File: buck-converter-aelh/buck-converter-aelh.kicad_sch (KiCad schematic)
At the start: 28 parts

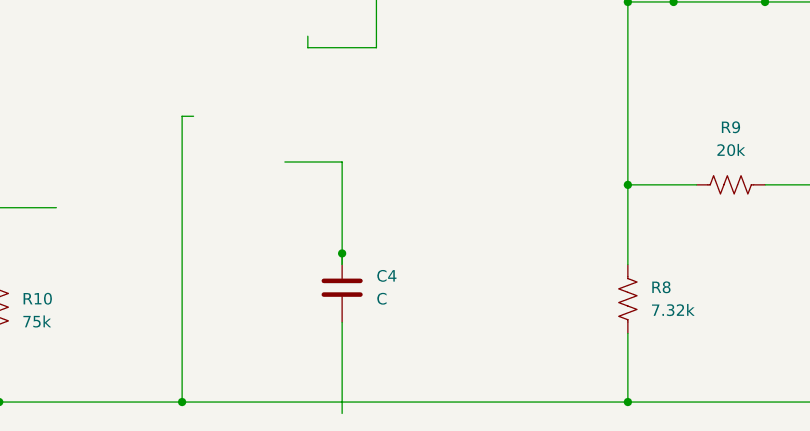
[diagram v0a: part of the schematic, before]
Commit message: AELH symbol
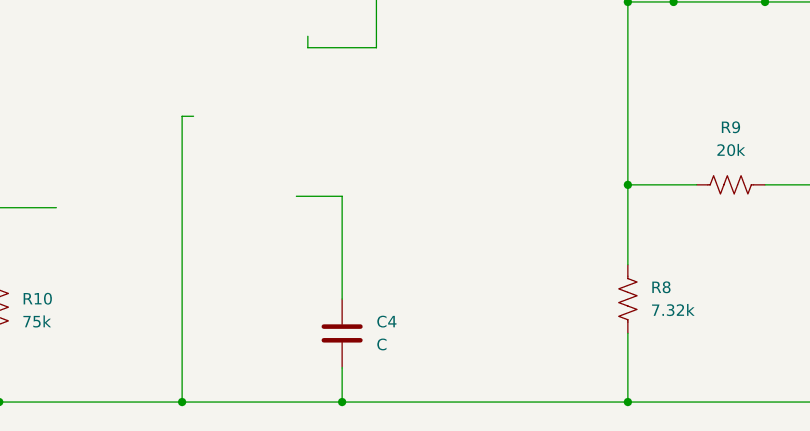
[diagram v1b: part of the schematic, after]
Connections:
- net at C1.2, C2.2, GND.1 (Pin_1)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: now also C4.2
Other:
- moved on the sheet: C4
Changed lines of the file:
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@@
   (junction (at 186.69 40.64) (diameter 0) (color 0 0 0 0)
   )
+  (junction (at 129.54 119.38) (diameter 0) (color 0 0 0 0)
+  )
   (junction (at 64.77 40.64) (diameter 0) (color 0 0 0 0)
   )
@@
   (junction (at 111.76 119.38) (diameter 0) (color 0 0 0 0)
   )
-  (junction (at 129.54 102.87) (diameter 0) (color 0 0 0 0)
-  )
   (junction (at 196.85 74.93) (diameter 0) (color 0 0 0 0)
   )
@@
     (stroke (width 0) (type default))
   )
-  (wire (pts (xy 129.54 110.49) (xy 129.54 120.65))
-    (stroke (width 0) (type default))
-  )
   (wire (pts (xy 207.01 67.31) (xy 207.01 74.93))
     (stroke (width 0) (type default))
@@
     (stroke (width 0) (type default))
   )
-  (wire (pts (xy 129.54 102.87) (xy 129.54 92.71))
-    (stroke (width 0) (type default))
-  )
   (wire (pts (xy 125.73 80.01) (xy 125.73 78.74))
     (stroke (width 0) (type default))
@@
     (stroke (width 0) (type default))
   )
-  (wire (pts (xy 129.54 104.14) (xy 129.54 102.87))
+  (wire (pts (xy 129.54 96.52) (xy 129.54 107.95))
     (stroke (width 0) (type default))
   )
@@
     (stroke (width 0) (type default))
   )
+  (wire (pts (xy 129.54 119.38) (xy 161.29 119.38))
+    (stroke (width 0) (type default))
+  )
   (wire (pts (xy 176.53 74.93) (xy 186.69 74.93))
     (stroke (width 0) (type default))
@@
     (stroke (width 0) (type default))
   )
-  (wire (pts (xy 111.76 119.38) (xy 161.29 119.38))
+  (wire (pts (xy 111.76 119.38) (xy 129.54 119.38))
     (stroke (width 0) (type default))
   )
@@
     (stroke (width 0) (type default))
   )
+  (wire (pts (xy 129.54 115.57) (xy 129.54 119.38))
+    (stroke (width 0) (type default))
+  )
   (wire (pts (xy 91.44 113.03) (xy 91.44 119.38))
     (stroke (width 0) (type default))
   )
-  (wire (pts (xy 129.54 92.71) (xy 123.19 92.71))
-    (stroke (width 0) (type default))
-  )
   (wire (pts (xy 217.17 74.93) (xy 227.33 74.93))
     (stroke (width 0) (type default))
@@
   )
   (wire (pts (xy 156.21 40.64) (xy 176.53 40.64))
+    (stroke (width 0) (type default))
+  )
+  (wire (pts (xy 129.54 96.52) (xy 124.46 96.52))
     (stroke (width 0) (type default))
   )
@@
     )
   )
-  (symbol (lib_id "Device:C") (at 129.54 106.68 0) (unit 1)
+  (symbol (lib_id "Device:C") (at 129.54 111.76 0) (unit 1)
     (in_bom yes) (on_board yes) (dnp no) (fields_autoplaced)
-    (property "Reference" "C4" (at 133.35 105.41 0)
-      (effects (font (size 1.27 1.27)) (justify left))
-    )
-    (property "Value" "C" (at 133.35 107.95 0)
-      (effects (font (size 1.27 1.27)) (justify left))
-    )
-    (property "Footprint" "" (at 130.5052 110.49 0)
-      (effects (font (size 1.27 1.27)) hide)
-    )
-    (property "Datasheet" "~" (at 129.54 106.68 0)
-      (effects (font (size 1.27 1.27)) hide)
-    )
+    (property "Reference" "C4" (at 133.35 110.49 0)
+      (effects (font (size 1.27 1.27)) (justify left))
+    )
+    (property "Value" "C" (at 133.35 113.03 0)
+      (effects (font (size 1.27 1.27)) (justify left))
+    )
+    (property "Footprint" "" (at 130.5052 115.57 0)
+      (effects (font (size 1.27 1.27)) hide)
+    )
+    (property "Datasheet" "~" (at 129.54 111.76 0)
+      (effects (font (size 1.27 1.27)) hide)
+    )

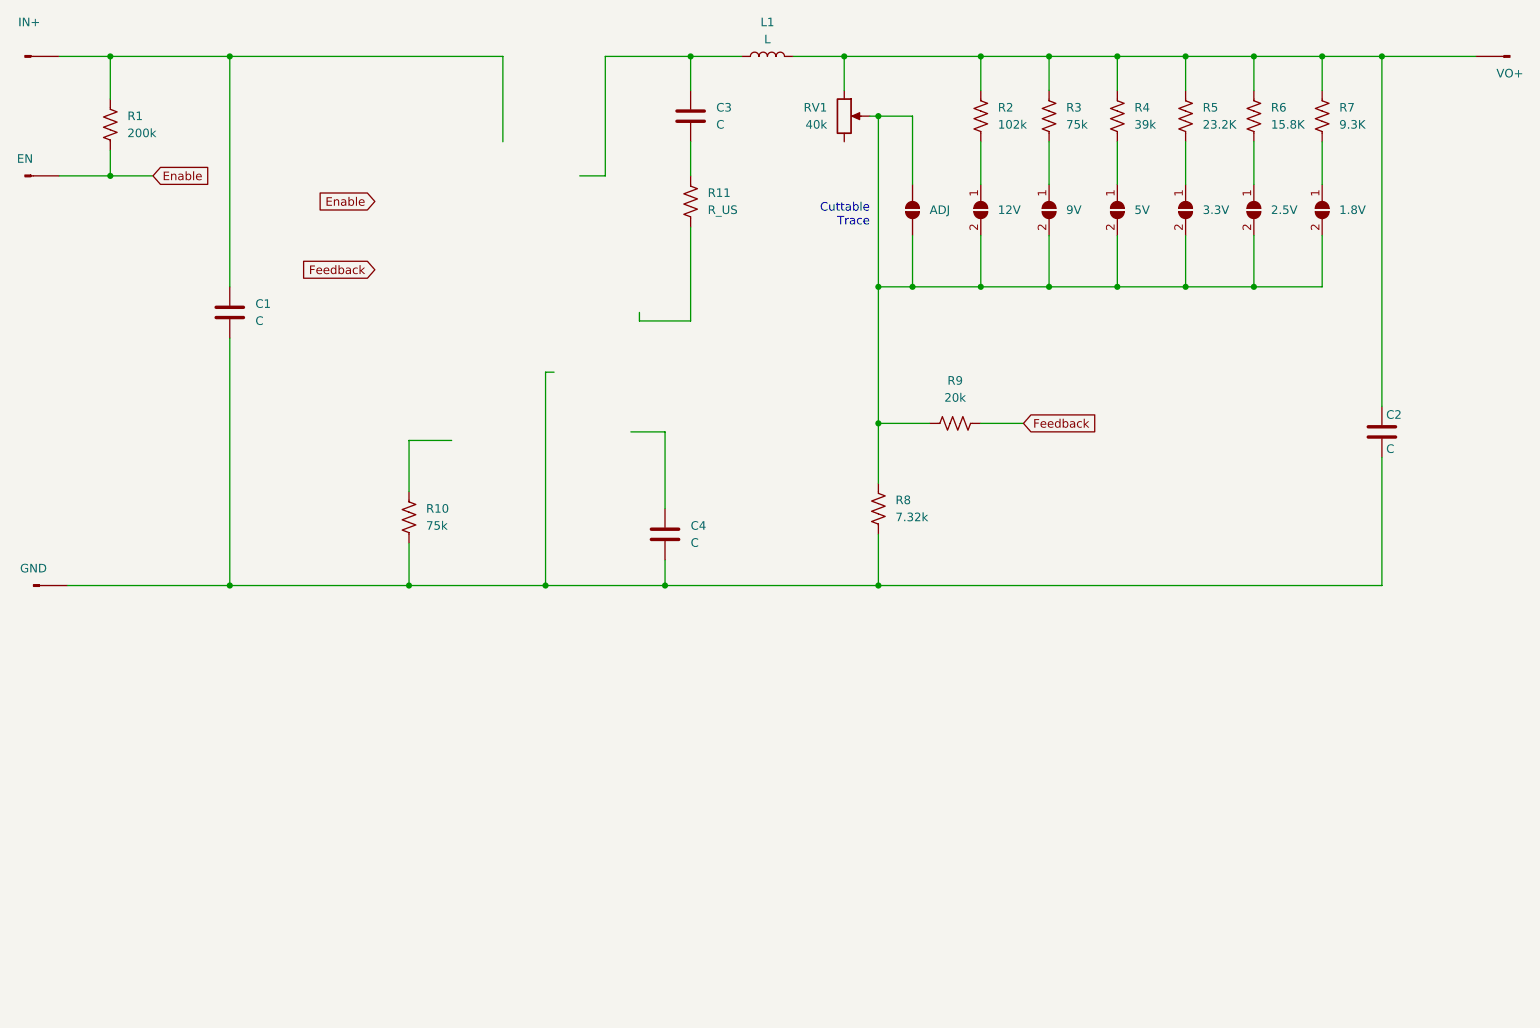
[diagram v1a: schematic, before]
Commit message: Tighten up layout and add notes
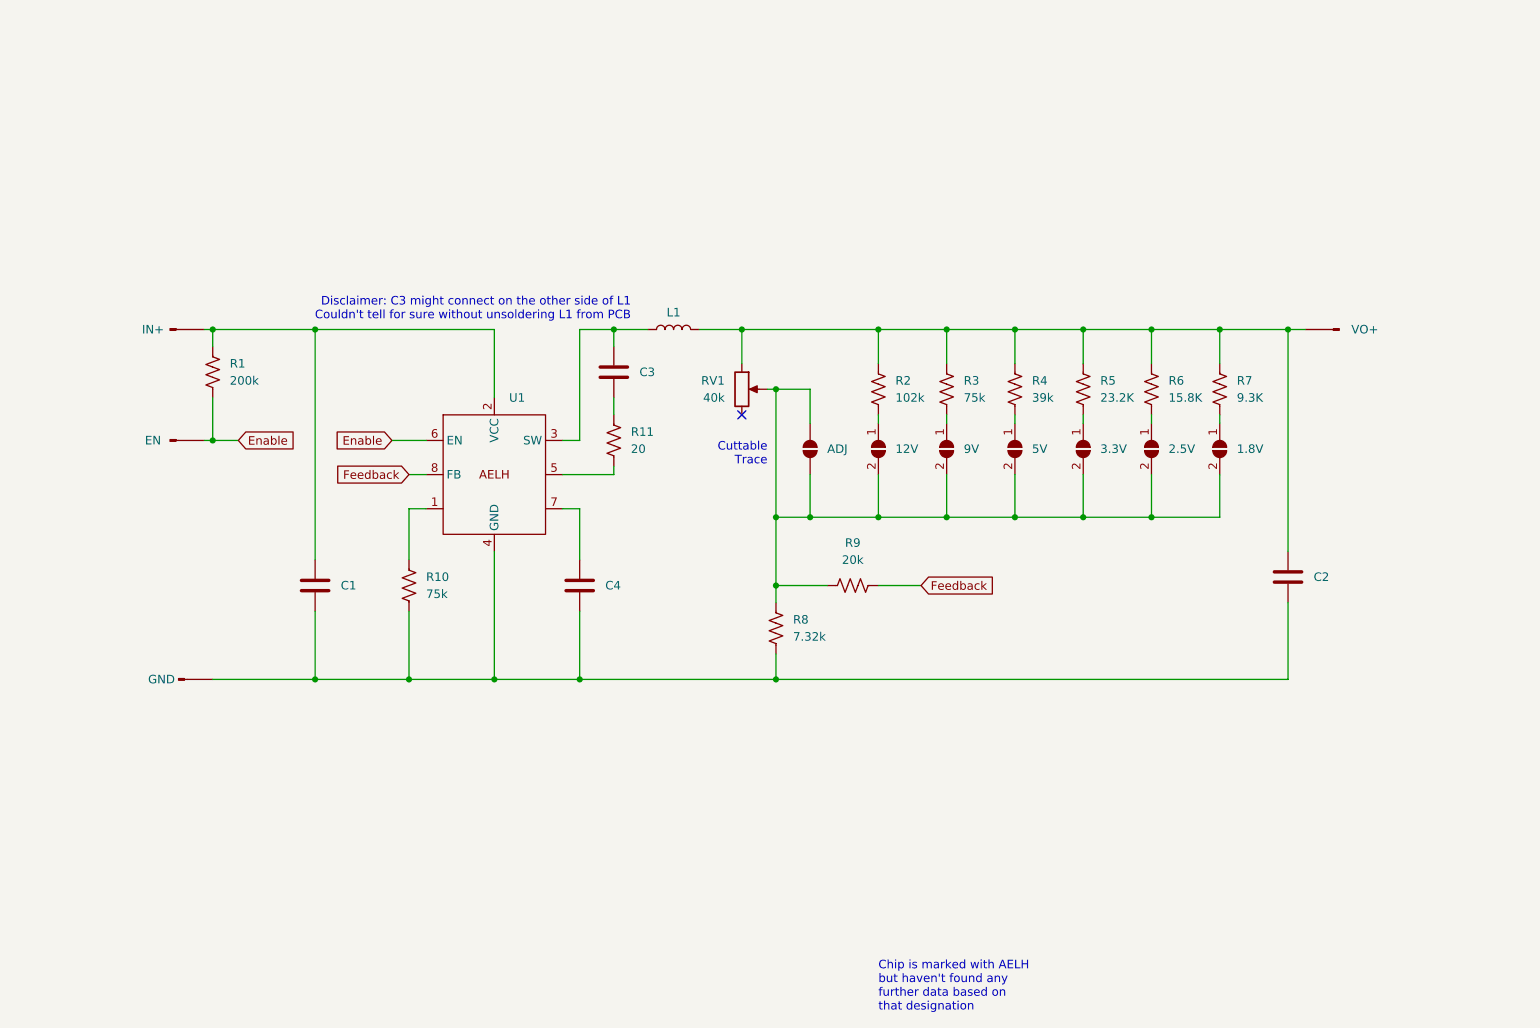
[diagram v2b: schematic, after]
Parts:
- added U1: ~, symbol aelh:AELH
- R11: value R_US -> 20
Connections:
- net Enable: now also U1.6 (EN)
- net Feedback: now also U1.8 (FB)
- net at C3.1, L1.1: now also U1.3 (SW)
- net at C1.2, C2.2, C4.2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: now also U1.4 (GND)
- net at C4.1: now also U1.7
- net at C1.1, IN+.1 (Pin_1), R1.1: now also U1.2 (VCC)
- net at R11.2: now also U1.5
- net at R10.2: now also U1.1
- no-connect marks 0 -> 1
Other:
- note added: "Chip is marked with AELH but haven't found any further data based on that designation"
- note added: "Disclaimer: C3 might connect on the other side of L1 Couldn't tell for sure without unsoldering L1 from PCB"
- moved on the sheet: ADJ, C1, C2, C3, C4, EN, GND, IN+, L1, R1, R10, R11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
